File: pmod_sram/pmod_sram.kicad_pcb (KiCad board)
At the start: 2 copper layers, 15.9 x 17.8 mm, 4 parts, among them J1 PMOD connector, U1 SRAM 1MB 20MHZ 1.8-5.5V

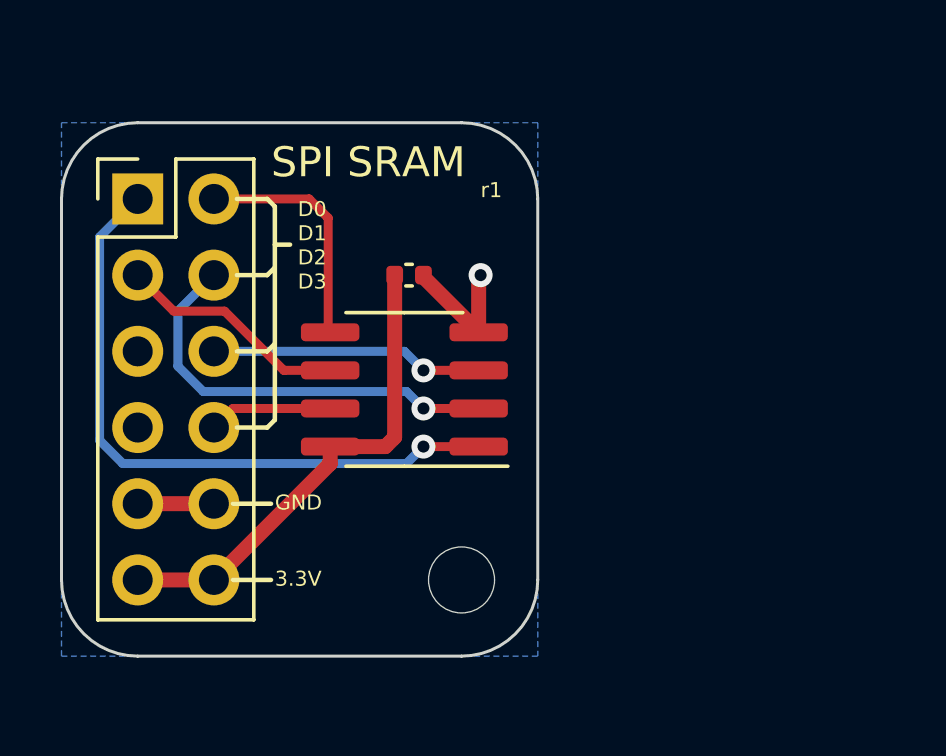
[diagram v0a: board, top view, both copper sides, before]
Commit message: New versions of PCB
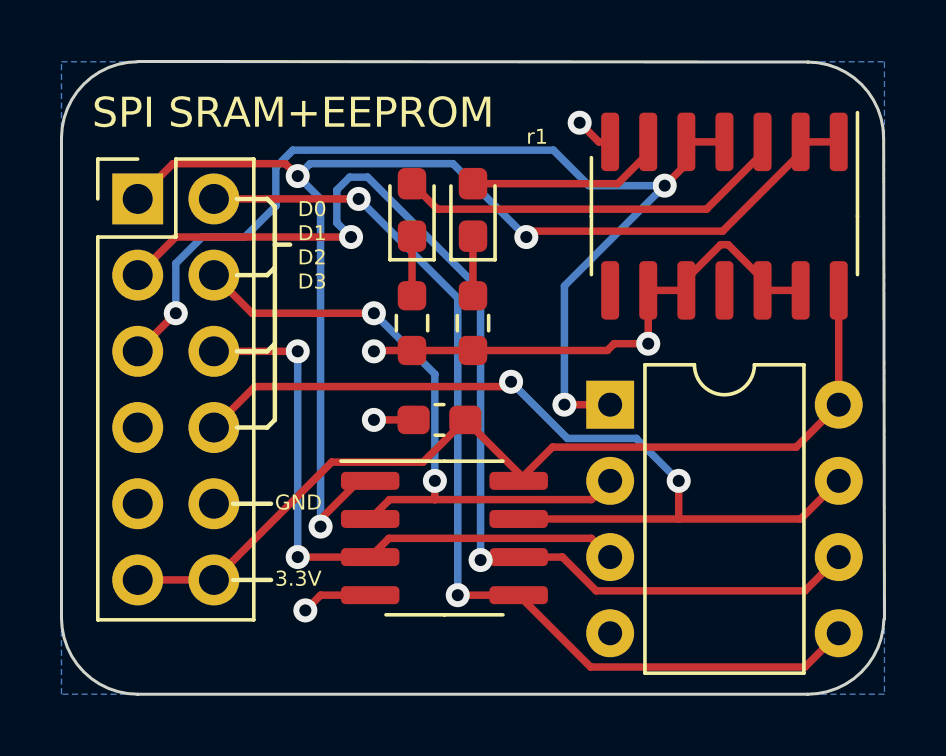
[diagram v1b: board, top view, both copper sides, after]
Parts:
- removed H1: MountingHole_Pad, MountingHole:MountingHole_2.2mm_M2
- added D1: LED, LED_SMD:LED_0603_1608Metric_Pad1.05x0.95mm_HandSolder, F.Cu at (72.6, 42.3)
- added D2: LED, LED_SMD:LED_0603_1608Metric_Pad1.05x0.95mm_HandSolder, F.Cu at (74.7, 42.3)
- added R1: R, Resistor_SMD:R_0603_1608Metric_Pad0.98x0.95mm_HandSolder, F.Cu at (72.6, 46.0)
- added R2: R, Resistor_SMD:R_0603_1608Metric_Pad0.98x0.95mm_HandSolder, F.Cu at (74.7, 46.0)
- added U2: 25LC1024 (DIP8 socket), Package_DIP:DIP-8_W7.62mm, F.Cu at (79.2, 48.8)
- added U3: 74HC00, Package_SO:SOIC-14_3.9x8.7mm_P1.27mm, F.Cu at (83.1, 42.5)
- C1: footprint Capacitor_SMD:C_0402_1005Metric -> Capacitor_SMD:C_0603_1608Metric_Pad1.08x0.95mm_HandSolder
- moved U1 5.13 mm to (73.7, 53.2), turned to 0 degrees
- moved C1 4.93 mm to (73.6, 49.3), turned to 180 degrees
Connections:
- net ~{CS} renamed ~{CS_SRAM}
- J1 pad 5: unconnected-(J1-Pin_5-Pad5) -> ~{CS_EEPROM}
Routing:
- net ~{CS_EEPROM}: track 0.00 -> 35.8 mm, vias 0 -> 3
- net SCK: track 7.73 -> 37.8 mm, vias 0 -> 2
- net D3: track 4.14 -> 30.0 mm, vias 0 -> 2
- net D0: track 7.91 -> 33.6 mm, vias 0 -> 2
- net ~{CS_SRAM}: track 21.8 -> 41.2 mm, vias 1 -> 3
- net GND: track 7.14 -> 22.8 mm, vias 1 -> 5
- net +3.3V: track 16.3 -> 31.4 mm
- net Net-(D1-A): track 0.00 -> 13.2 mm
- net D2: track 9.09 -> 20.6 mm, vias 1 -> 2
- net D1: track 14.1 -> 21.4 mm, vias 1 -> 2
- net Net-(D2-A): track 0.00 -> 6.64 mm
- net Net-(D2-K): track 0.00 -> 1.98 mm
- net Net-(D1-K): track 0.00 -> 1.98 mm
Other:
- board size 15.9 x 17.8 mm -> 27.4 x 21.1 mm
- board text added: "SPI SRAM+EEPROM"
- board text added: "~{EEPROM_CS}"
- board text added: "~{SRAM_CS}"
- board text removed: "SPI SRAM"
- board text removed: "~{CS}"
